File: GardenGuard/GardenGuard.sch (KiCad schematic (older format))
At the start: 52 parts, among them J1 Sollar, J2 OLED SSD1306, J3 AudioJack4_Ground_SwitchTR1, Q3 FQP27P06, SW1 Reset, SW2 SW_Push, SW3 Rotary_Encoder_Switch, U1 ESP-07, U2 DS18B20, U4 TP4056, U5 FS8205A, U6 DW01A, U7 HT75xx-1-SOT89

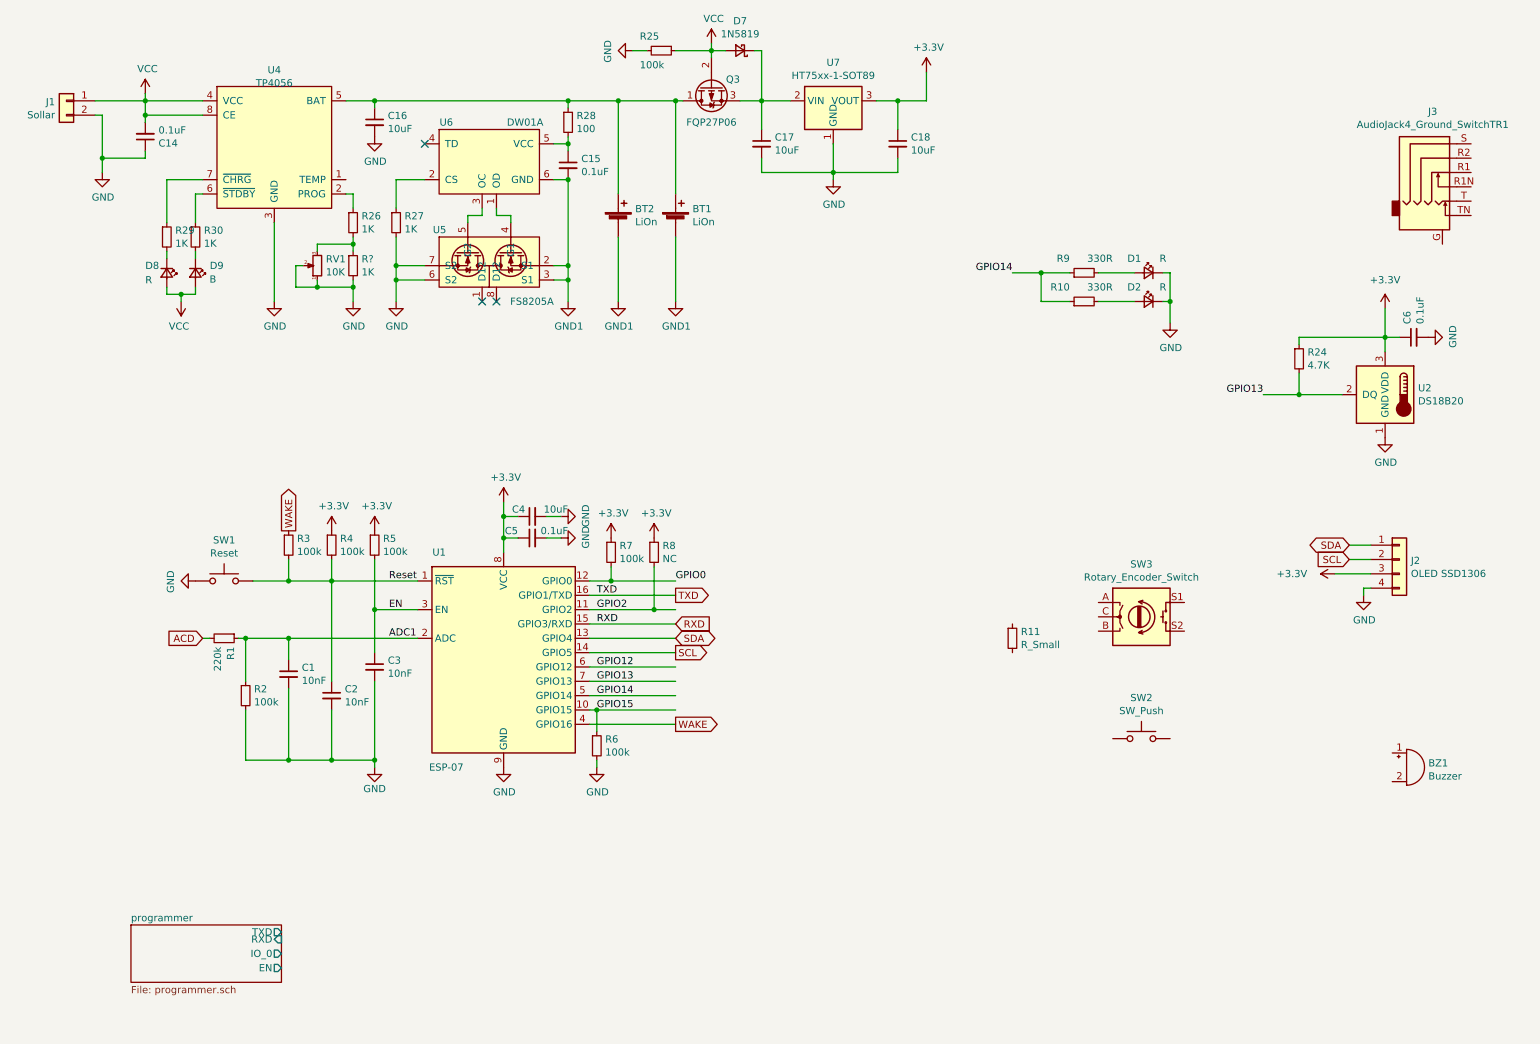
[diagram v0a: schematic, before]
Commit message: shematic finished
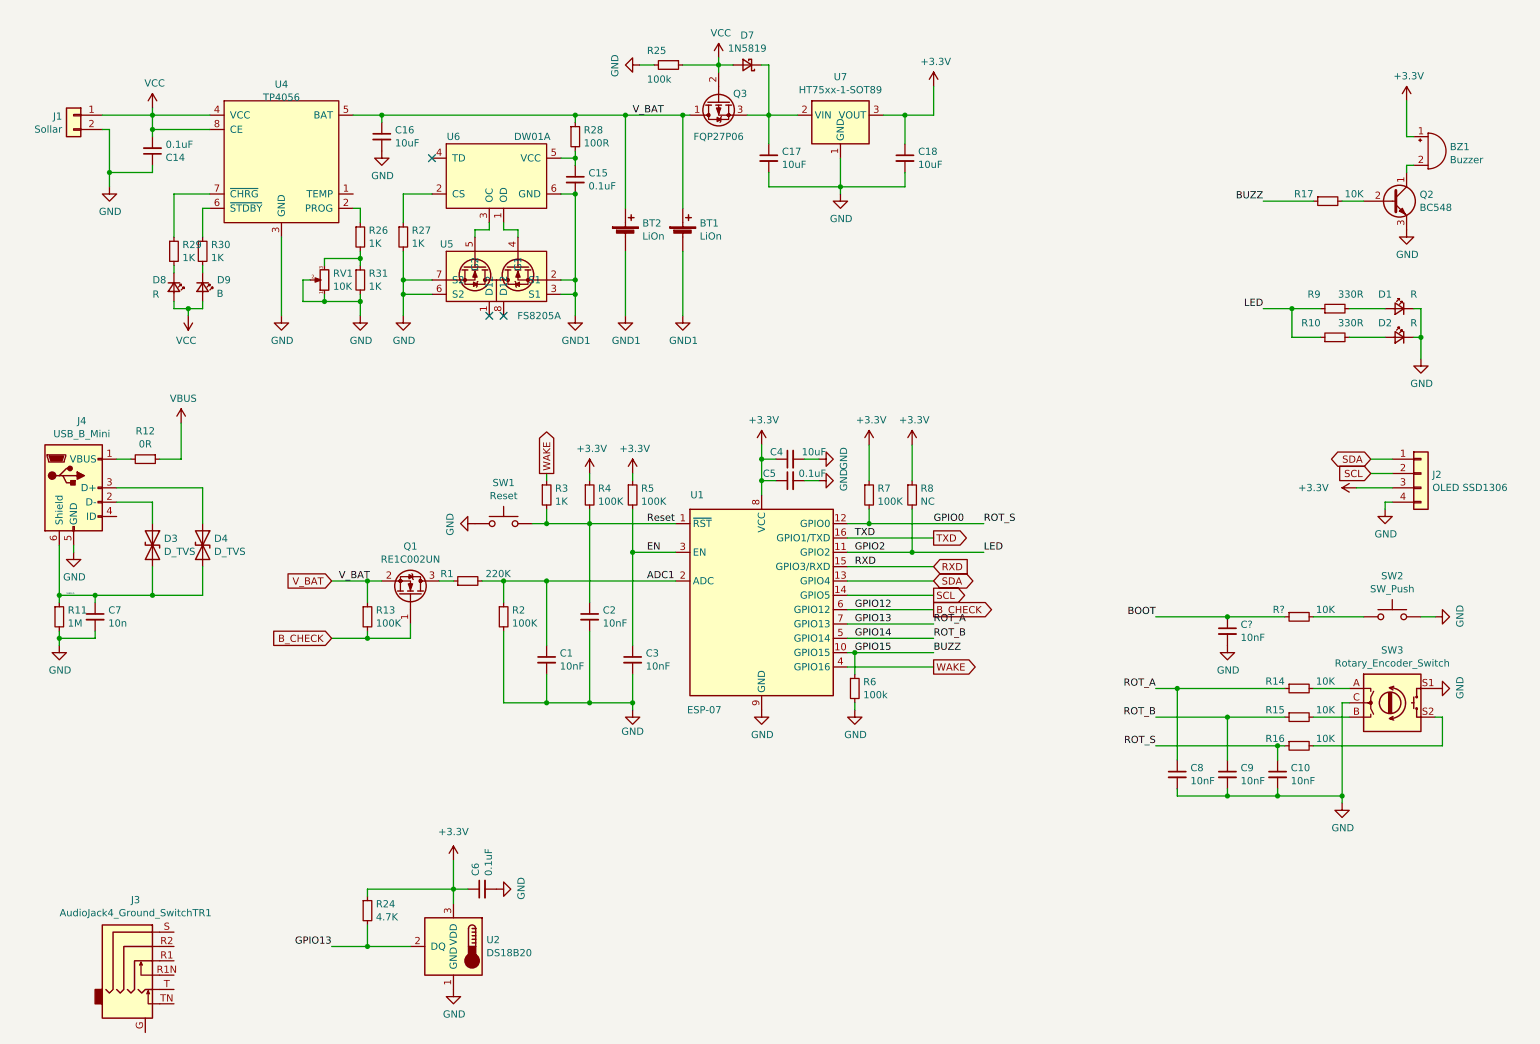
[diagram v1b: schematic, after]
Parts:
- added C10, C8, C9, C?: 10nF, Capacitor_SMD:C_0805_2012Metric_Pad1.18x1.45mm_HandSolder, symbol Device:C_Small
- added C7: 10n, Capacitor_SMD:C_0805_2012Metric_Pad1.18x1.45mm_HandSolder, symbol Device:C_Small
- added D3, D4: D_TVS, Diode_SMD:D_0805_2012Metric_Castellated, symbol Device:D_TVS
- added J4: USB_B_Mini, Connector_USB:USB_Micro-B_Amphenol_10118194_Horizontal, symbol Connector:USB_B_Mini
- added Q1: RE1C002UN, symbol Device:Q_NMOS_GSD
- added Q2: BC548, Package_TO_SOT_THT:TO-92_Inline, symbol Transistor_BJT:BC548
- added R12: 0R, Resistor_SMD:R_0805_2012Metric_Pad1.20x1.40mm_HandSolder, symbol Device:R_Small
- added R13: 100K, Resistor_SMD:R_0805_2012Metric_Pad1.20x1.40mm_HandSolder, symbol Device:R_Small
- added R14, R15, R16, R17, R?: 10K, Resistor_SMD:R_0805_2012Metric_Pad1.20x1.40mm_HandSolder, symbol Device:R_Small
- R1: value 220k -> 220K
- R11: value R_Small -> 1M
- R2, R4, R5, R7: value 100k -> 100K
- R28: value 100 -> 100R
- R3: value 100k -> 1K
- gave numbers to parts that had none: 1
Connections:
- net labels added: BOOT, BUZZ, B_CHECK, LED, ROT_A, ROT_B, ROT_S, SHIELD, VBUS, V_BAT
- net labels removed: ACD
- wire segments 160 -> 225
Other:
- moved on the sheet: BT1, BT2, BZ1, C1, C14, C15, C16, C17, C18, C2, C3, C4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
